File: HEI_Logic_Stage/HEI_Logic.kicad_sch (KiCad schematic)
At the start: 46 parts, among them J5 Tag-Connect, SW1 SW_Push, U6 STM32F334C8T6, U7 LM4132-Q1 SOT-2

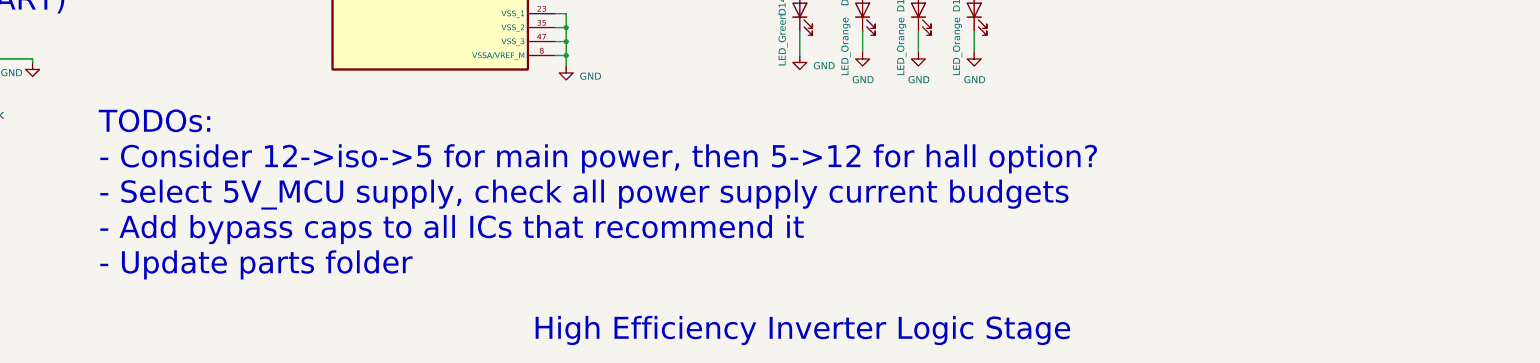
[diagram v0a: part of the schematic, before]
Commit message: more minor updates
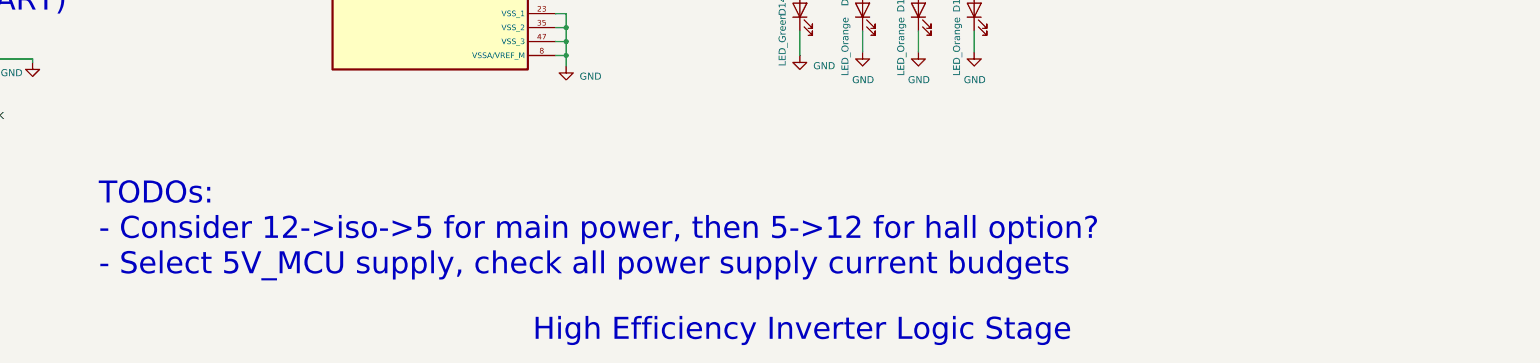
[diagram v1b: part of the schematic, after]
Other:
- note added: "TODOs: - Consider 12->iso->5 for main power, then 5->12 for hall option? - Select 5V_MCU supply, check all power supply current budgets"
- note removed: "TODOs: - Consider 12->iso->5 for main power, then 5->12 for hall option? - Select 5V_MCU supply, check all power supply current budgets - Add bypass caps to all ICs that recommend it - Update parts folder"
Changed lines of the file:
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@@
 		)
 	)
-	(text "TODOs:\n- Consider 12->iso->5 for main power, then 5->12 for hall option?\n- Select 5V_MCU supply, check all power supply current budgets\n- Add bypass caps to all ICs that recommend it\n- Update parts folder"
+	(text "TODOs:\n- Consider 12->iso->5 for main power, then 5->12 for hall option?\n- Select 5V_MCU supply, check all power supply current budgets"
 		(exclude_from_sim no)
 		(at 101.6 164.846 0)
